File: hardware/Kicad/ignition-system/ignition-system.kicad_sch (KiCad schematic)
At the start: 3 parts, among them U1 SX1278, U2 RP2040

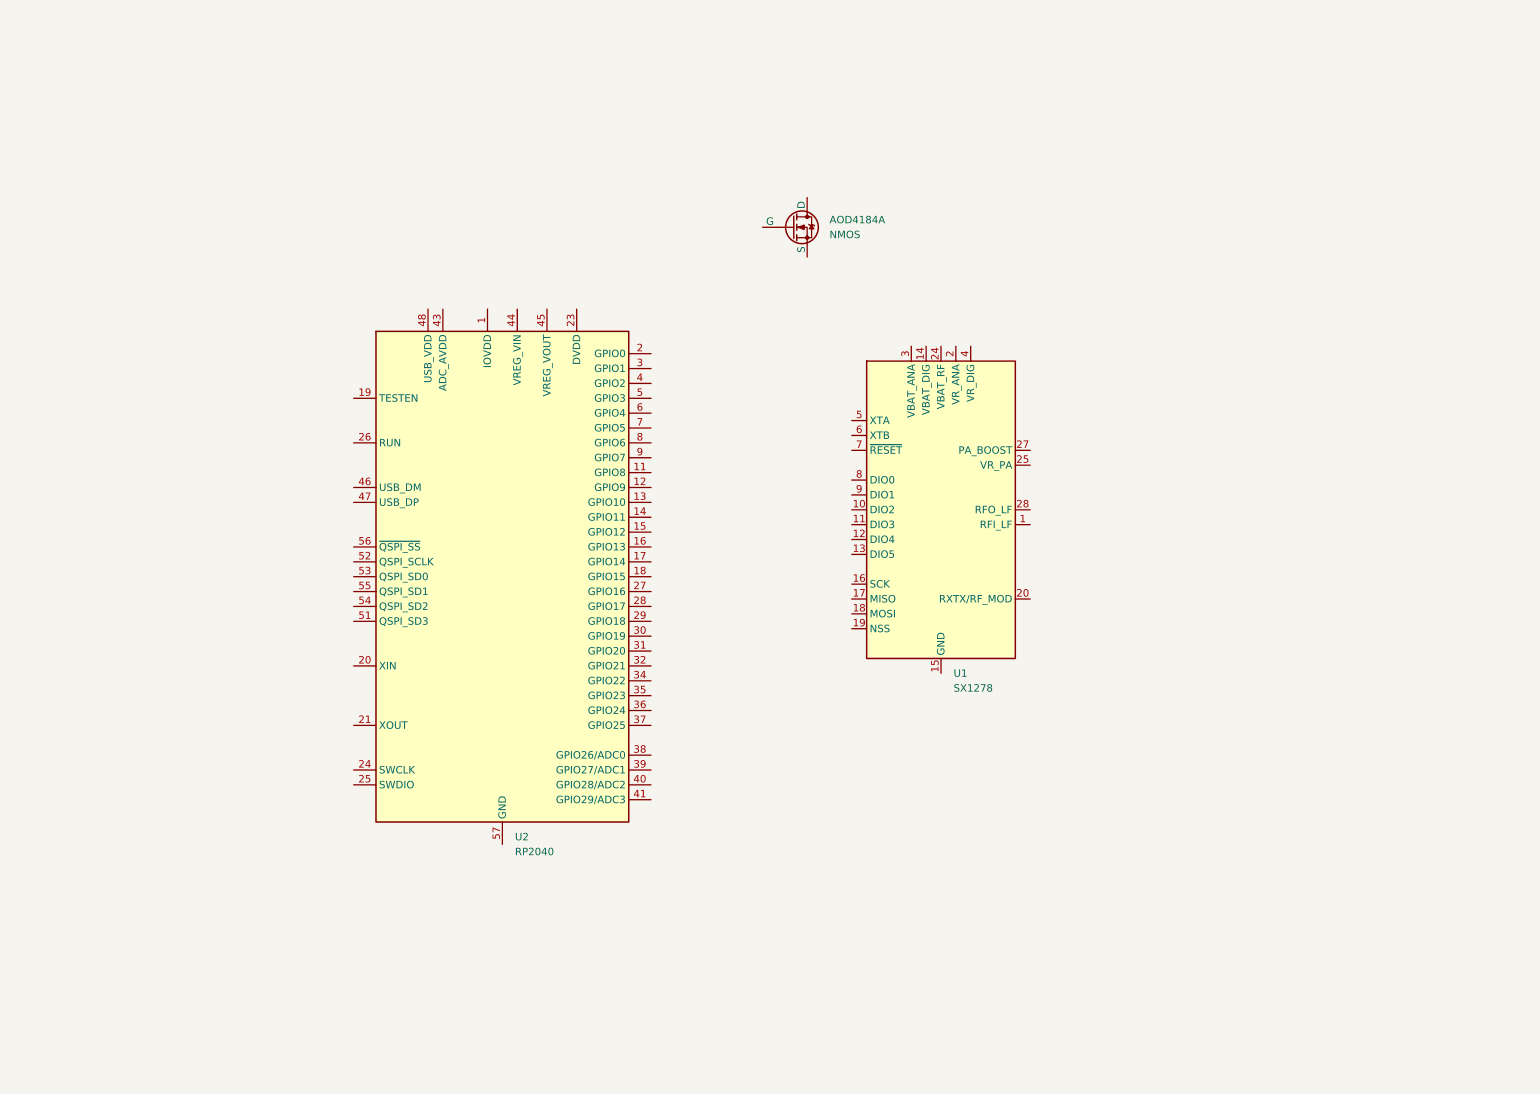
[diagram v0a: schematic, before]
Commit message: feat: nuevos componentes y estructura con net labels
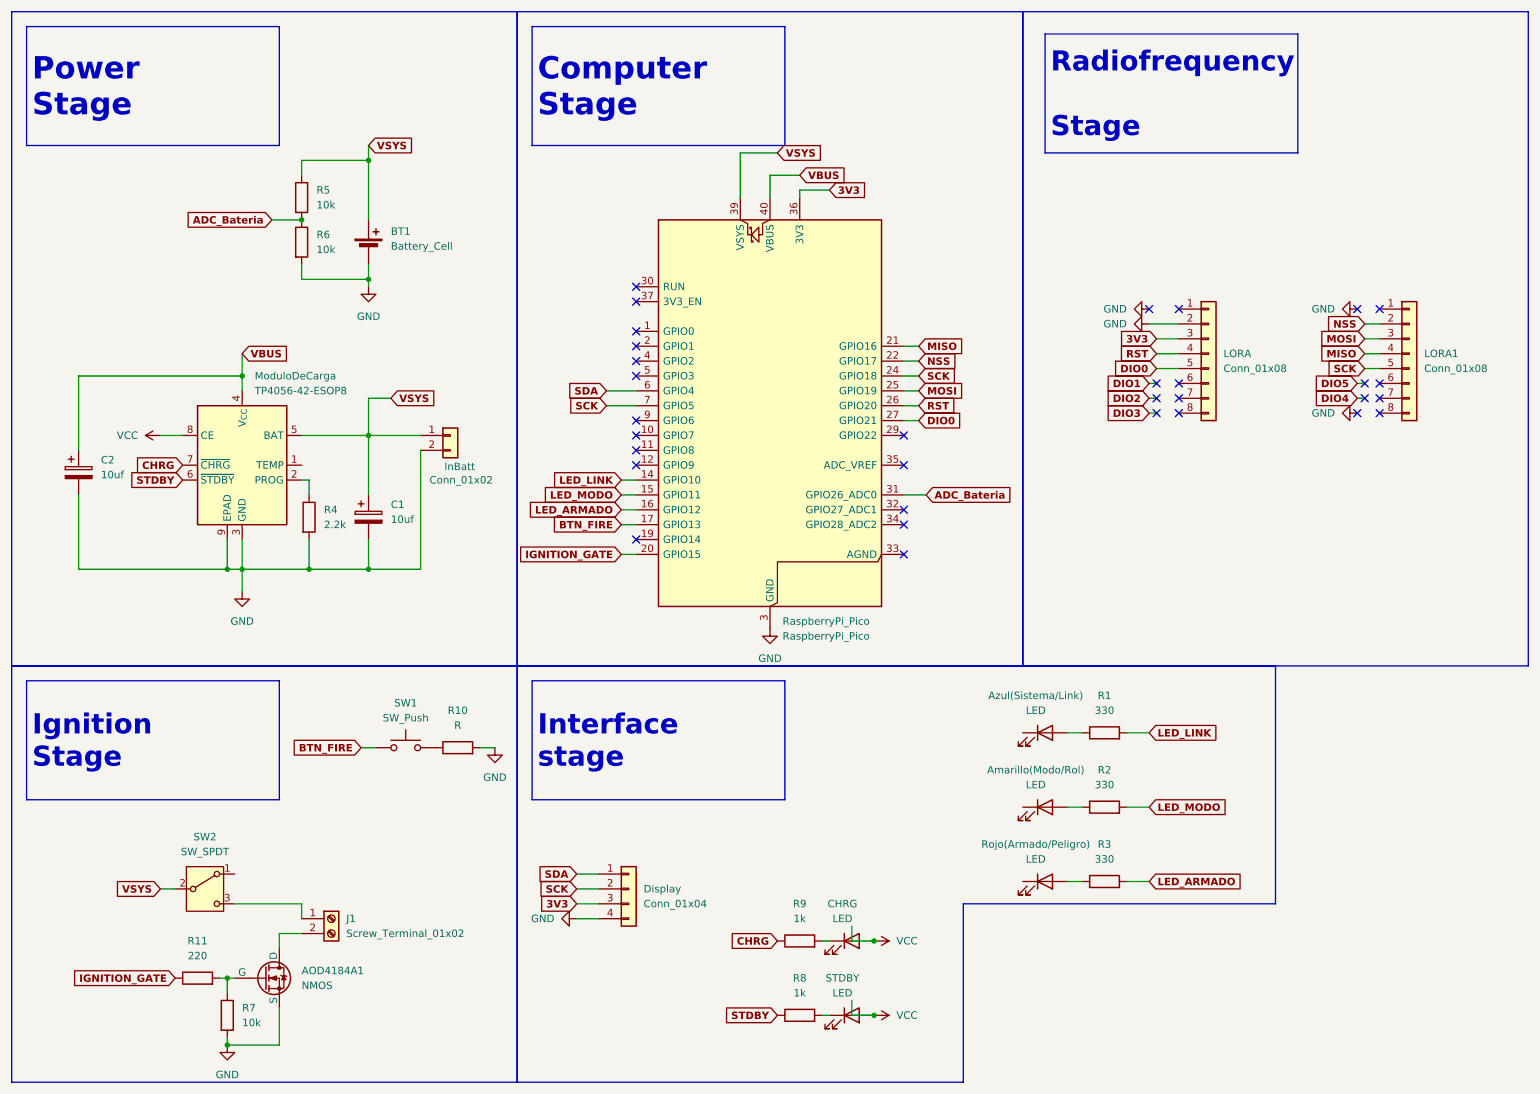
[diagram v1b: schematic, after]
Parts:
- removed U1: SX1278, Package_DFN_QFN:QFN-28-1EP_6x6mm_P0.65mm_EP4.8x4.8mm, symbol RF:SX1278
- removed U2: RP2040, Package_DFN_QFN:QFN-56-1EP_7x7mm_P0.4mm_EP3.2x3.2mm, symbol MCU_RaspberryPi:RP2040
- added Amarillo(Modo/Rol), Azul(Sistema/Link), CHRG, Rojo(Armado/Peligro), STDBY: LED, LED_SMD:LED_0805_2012Metric, symbol Device:LED
- added BT1: Battery_Cell, symbol Device:Battery_Cell
- added C1, C2: 10uf, symbol Device:C_Polarized
- added Display: Conn_01x04, symbol Connector_Generic:Conn_01x04
- added InBatt: Conn_01x02, Connector_JST:JST_PH_S2B-PH-K_1x02_P2.00mm_Horizontal, symbol Connector_Generic:Conn_01x02
- added J1: Screw_Terminal_01x02, symbol Connector:Screw_Terminal_01x02
- added LORA, LORA1: Conn_01x08, symbol Connector_Generic:Conn_01x08
- added ModuloDeCarga: TP4056-42-ESOP8, Package_SO:SOIC-8-1EP_3.9x4.9mm_P1.27mm_EP2.41x3.3mm_ThermalVias, symbol Battery_Management:TP4056-42-ESOP8
- added R1, R2, R3: 330, symbol Device:R
- added R10: R, symbol Device:R
- added R11: 220, symbol Device:R
- added R4: 2.2k, symbol Device:R
- added R5, R6, R7: 10k, symbol Device:R
- added R8, R9: 1k, symbol Device:R
- added RaspberryPi_Pico: RaspberryPi_Pico, Module:RaspberryPi_Pico_Common_Unspecified, symbol MCU_Module:RaspberryPi_Pico
- added SW1: SW_Push, symbol Switch:SW_Push
- added SW2: SW_SPDT, symbol Switch:SW_SPDT
- renumbered AOD4184A to AOD4184A1
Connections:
- net at AOD4184A1.1 (D): now also J1.2 (Pin_2)
- net at AOD4184A1.2 (G): now also R11.2, R7.1
- net GND: now reaches AOD4184A1.3 (S)
- net GND: now also BT1.2 (-), C1.2, C2.2, Display.4 (Pin_4), InBatt.2 (Pin_2), LORA.2 (Pin_2), ModuloDeCarga.3 (GND), ModuloDeCarga.9 (EPAD), R10.2, R4.2, R6.2, R7.2, RaspberryPi_Pico.13 (GND), RaspberryPi_Pico.18 (GND), RaspberryPi_Pico.23 (GND), RaspberryPi_Pico.28 (GND), RaspberryPi_Pico.3 (GND), RaspberryPi_Pico.38 (GND), RaspberryPi_Pico.8 (GND)
- new net: R10.1, SW1.2
- new net: CHRG.1 (K), R9.2
- new net: R3.1, Rojo(Armado/Peligro).2 (A)
- new net: Azul(Sistema/Link).2 (A), R1.1
- new net: R8.2, STDBY.1 (K)
- new net: J1.1 (Pin_1), SW2.3 (C)
- new net: ModuloDeCarga.2 (PROG), R4.1
- new net: Amarillo(Modo/Rol).2 (A), R2.1
- new net 3V3: Display.3 (Pin_3), LORA.3 (Pin_3), RaspberryPi_Pico.36 (3V3)
- new net ADC_Bateria: R5.2, R6.1, RaspberryPi_Pico.31 (GPIO26_ADC0)
- new net BTN_FIRE: RaspberryPi_Pico.17 (GPIO13), SW1.1
- new net CHRG: ModuloDeCarga.7 (~{CHRG}), R9.1
- new net DIO0: LORA.5 (Pin_5), RaspberryPi_Pico.27 (GPIO21)
- new net IGNITION_GATE: R11.1, RaspberryPi_Pico.20 (GPIO15)
- new net LED_ARMADO: R3.2, RaspberryPi_Pico.16 (GPIO12)
- new net LED_LINK: R1.2, RaspberryPi_Pico.14 (GPIO10)
- new net LED_MODO: R2.2, RaspberryPi_Pico.15 (GPIO11)
- new net MISO: LORA1.4 (Pin_4), RaspberryPi_Pico.21 (GPIO16)
- new net MOSI: LORA1.3 (Pin_3), RaspberryPi_Pico.25 (GPIO19)
- new net NSS: LORA1.2 (Pin_2), RaspberryPi_Pico.22 (GPIO17)
- new net RST: LORA.4 (Pin_4), RaspberryPi_Pico.26 (GPIO20)
- new net SCK: Display.2 (Pin_2), LORA1.5 (Pin_5), RaspberryPi_Pico.24 (GPIO18), RaspberryPi_Pico.7 (GPIO5)
- new net SDA: Display.1 (Pin_1), RaspberryPi_Pico.6 (GPIO4)
- new net STDBY: ModuloDeCarga.6 (~{STDBY}), R8.1
- new net VBUS: C2.1, ModuloDeCarga.4 (V_{CC}), RaspberryPi_Pico.40 (VBUS)
- new net VCC: CHRG.2 (A), ModuloDeCarga.8 (CE), STDBY.2 (A)
- new net VSYS: BT1.1 (+), C1.1, InBatt.1 (Pin_1), ModuloDeCarga.5 (BAT), R5.1, RaspberryPi_Pico.39 (VSYS), SW2.2 (B)
- no-connect marks 0 -> 32
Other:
- title: (none) -> Ignition Sistem
- moved on the sheet: AOD4184A1
